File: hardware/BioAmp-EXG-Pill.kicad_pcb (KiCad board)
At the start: 2 copper layers, 38 parts, among them J1 BioAmp Output, J2 BioAmp Input, U1 Amp, U2 LOGO_UDLABS

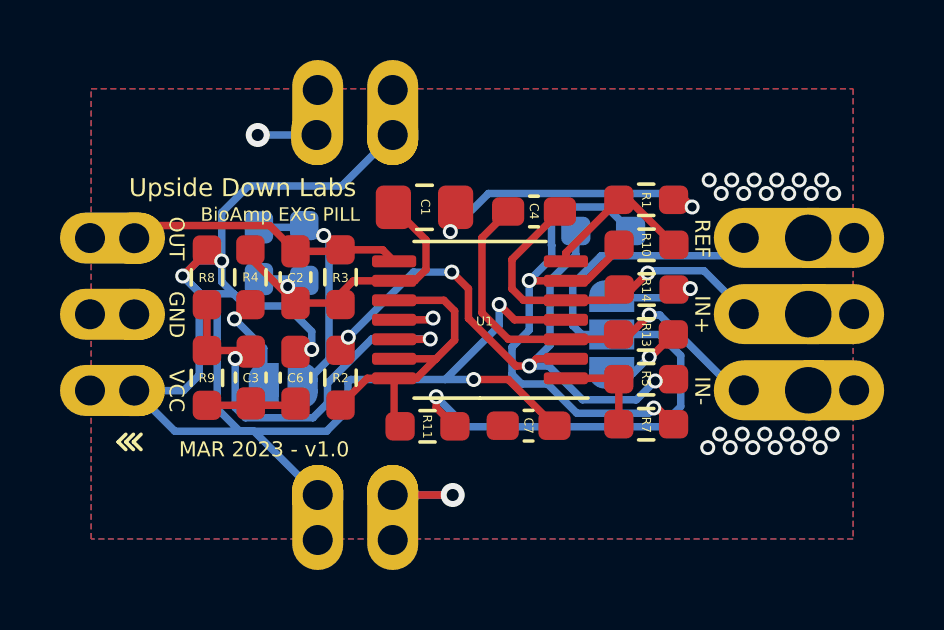
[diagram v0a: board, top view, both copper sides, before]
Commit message: add connectors and fill in ground
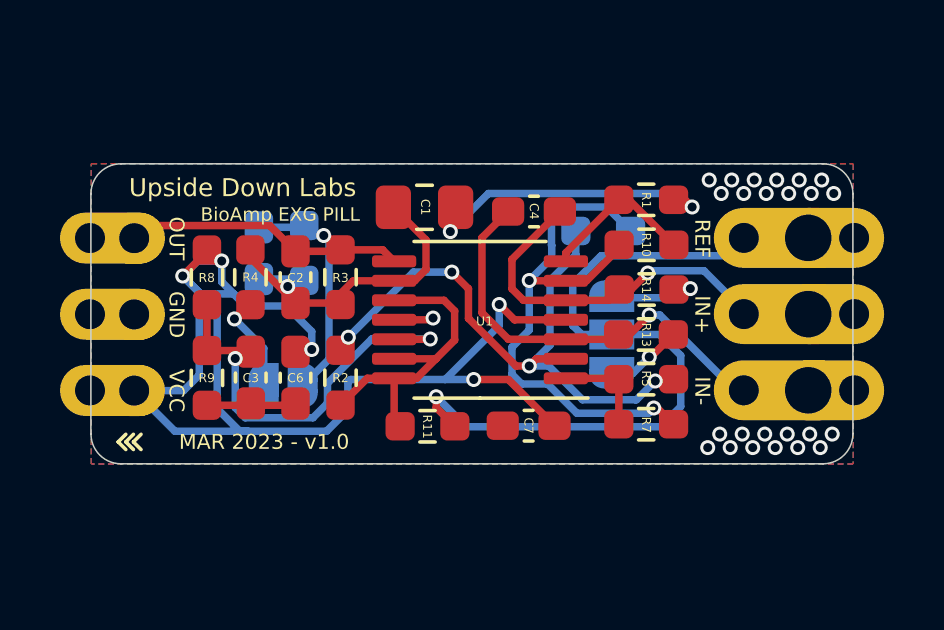
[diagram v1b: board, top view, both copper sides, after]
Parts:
- removed ? (x8): , 
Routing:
- net VCC: track 56.2 -> 44.6 mm
- net GND: track 10.2 -> 4.30 mm, vias 27 -> 25
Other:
- board outline added: 25.4 x 10 mm
